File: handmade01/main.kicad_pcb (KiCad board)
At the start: 2 copper layers, 64.8 x 70.1 mm, 71 parts, among them CON1 MicroSD, CON2 MicroSD, J1 JACK_TRS_6PINS, P1 VOLUMN, P4 USB_OTG, P6 UART_DEBUG, Q1 1AM, SW1 Power, SW10 R, SW11 A, SW12 B, SW13 X, SW14 Y, SW2 Reset, SW3 UP, SW4 Down, SW5 Left, SW6 Right, SW7 Select, SW8 Start, SW9 L, U1 PCM5102A, U2 PAM8403, U3 IPS_2.4_240x320_ST7789V, U4 CM3354, U5 TPS71718

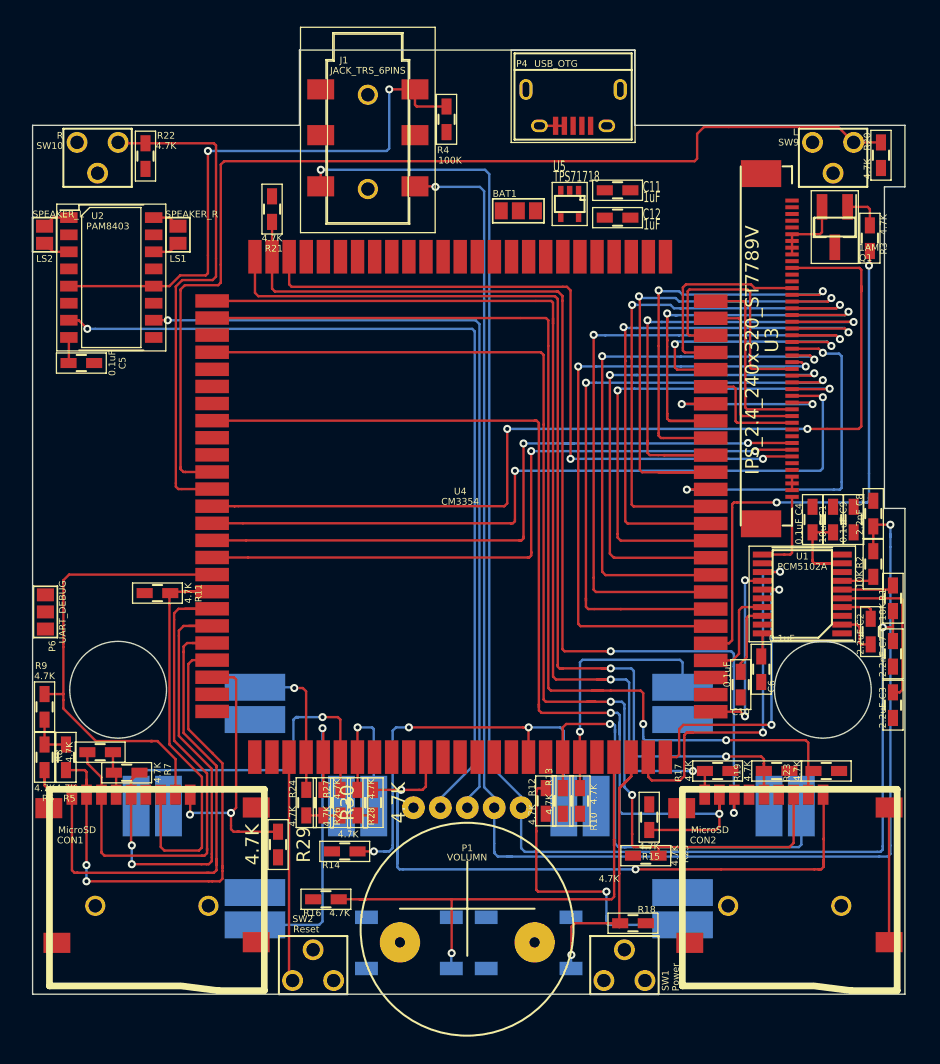
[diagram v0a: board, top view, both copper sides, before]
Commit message: 20171217
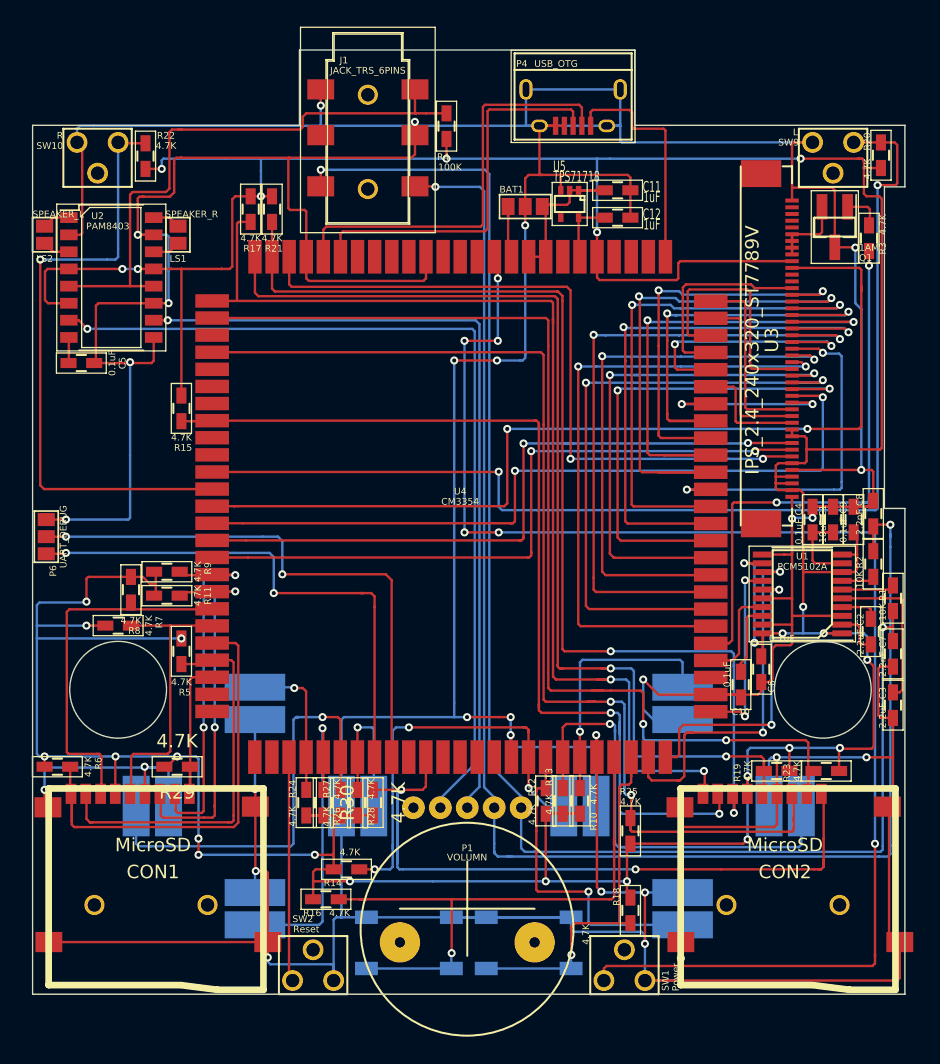
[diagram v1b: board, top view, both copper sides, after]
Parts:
- moved R17 54.2 mm to (126.7, 79.4), turned to 270 degrees
- moved R15 46.1 mm to (121.5, 94.2)
- moved R9 13.5 mm to (120.5, 106.3), turned to 0 degrees
- moved R8 12.3 mm to (117.8, 107.6), turned to 270 degrees
- moved R5 11.6 mm to (121.5, 112.2)
- moved R7 10.9 mm to (116.8, 110.3)
- moved R29 9.46 mm to (121.2, 120.8), turned to 180 degrees
- moved P6 5.59 mm to (111.5, 103.7)
- moved R25 2.17 mm to (154.9, 125.5), turned to 90 degrees
- moved R14 1.34 mm to (133.8, 128.4)
- moved R6 1.18 mm to (112.3, 120.8), turned to 0 degrees
- moved R18 0.97 mm to (154.9, 131.4), turned to 270 degrees
- moved R11 0.72 mm to (120.5, 108.1)
- moved BAT1 0.60 mm to (147.1, 79.2)
- moved R4 0.51 mm to (141.2, 73.2)
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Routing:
- net GND: track 28.6 -> 586.5 mm, vias 0 -> 29
- net +3.3V: track 14.4 -> 363.5 mm, vias 0 -> 29
- net POWER: track 0.00 -> 106.8 mm, vias 0 -> 6
- net UART_TX: track 0.00 -> 41.6 mm, vias 0 -> 2
- net UART_RX: track 0.00 -> 39.4 mm, vias 0 -> 2
- net USB_DM: track 0.00 -> 31.6 mm
- net USB_DP: track 0.00 -> 29.0 mm
- net +5V: track 0.00 -> 17.3 mm
- net SD0_CLK: track 35.6 -> 21.3 mm, vias 2 -> 0
- net SD0_CMD: track 39.8 -> 26.9 mm
- net BAT_+: track 0.00 -> 12.8 mm
- net SD0_DAT3: track 40.0 -> 28.8 mm, vias 2 -> 0
- net SD0_CD: track 21.4 -> 12.3 mm, vias 2 -> 0
- net SD0_DAT2: track 42.6 -> 34.2 mm
- net R: track 38.0 -> 46.1 mm, vias 0 -> 1
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
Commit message: 20171217
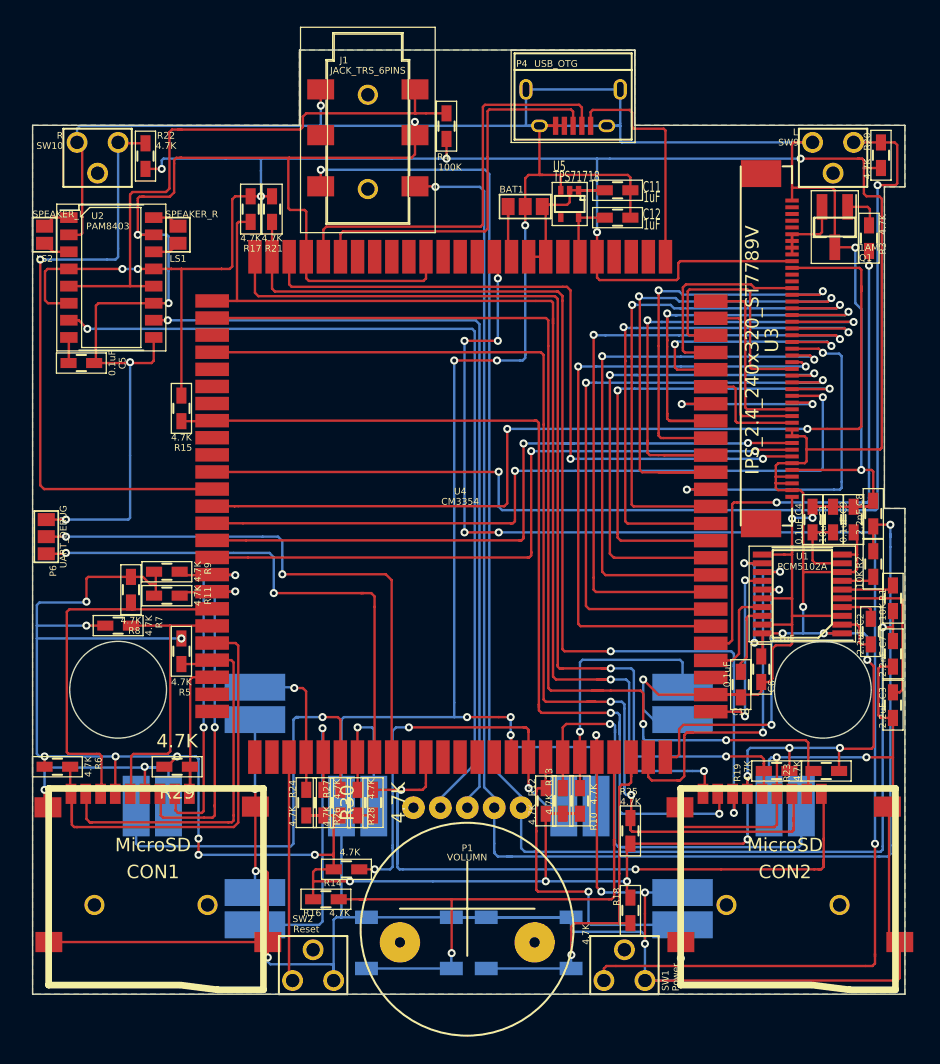
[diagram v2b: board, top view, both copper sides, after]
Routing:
- added copper zone on B.Cu, net GND
- added copper zone on F.Cu, net GND
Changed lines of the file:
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@@
   (page A4)
   (layers
-    (15 F.Cu signal)
-    (0 B.Cu signal)
-    (16 B.Adhes user)
-    (17 F.Adhes user)
-    (18 B.Paste user)
-    (19 F.Paste user)
-    (20 B.SilkS user)
-    (21 F.SilkS user)
-    (22 B.Mask user)
-    (23 F.Mask user)
-    (24 Dwgs.User user)
-    (25 Cmts.User user)
-    (26 Eco1.User user)
-    (27 Eco2.User user)
+    (15 F.Cu signal hide)
+    (0 B.Cu signal hide)
+    (16 B.Adhes user hide)
+    (17 F.Adhes user hide)
+    (18 B.Paste user hide)
+    (19 F.Paste user hide)
+    (20 B.SilkS user hide)
+    (21 F.SilkS user hide)
+    (22 B.Mask user hide)
+    (23 F.Mask user hide)
+    (24 Dwgs.User user hide)
+    (25 Cmts.User user hide)
+    (26 Eco1.User user hide)
+    (27 Eco2.User user hide)
     (28 Edge.Cuts user)
   )
@@
     (pad_to_mask_clearance 0)
     (aux_axis_origin 0 0)
-    (visible_elements 7FFFFFEF)
+    (visible_elements 7FFFFFFF)
     (pcbplotparams
       (layerselection 536838145)
@@
   (segment (start 134.62 122.494) (end 134.62 120.0731) (width 0.18) (layer F.Cu) (net 87))
   (segment (start 134.62 120.0731) (end 134.6098 120.0629) (width 0.18) (layer F.Cu) (net 87))
+  (zone (net 12) (net_name GND) (layer B.Cu) (hatch edge 0.508)
+    (connect_pads (clearance 0.18))
+    (min_thickness 0.18)
+    (fill (arc_segments 16) (thermal_gap 0.2) (thermal_bridge_width 0.2))
+    (polygon
+      (pts
+        (xy 175.26 137.668) (xy 110.49 137.668) (xy 110.49 73.152) (xy 130.302 73.152) (xy 130.302 67.564)
+        (xy 155.194 67.564) (xy 155.194 73.152) (xy 175.26 73.152) (xy 175.26 77.724) (xy 173.736 77.724)
+        (xy 173.736 101.6) (xy 175.26 101.6)
+      )
+    )
+  )
+  (zone (net 12) (net_name GND) (layer F.Cu) (hatch edge 0.508)
+    (connect_pads (clearance 0.18))
+    (min_thickness 0.18)
+    (fill (arc_segments 16) (thermal_gap 0.2) (thermal_bridge_width 0.2))
+    (polygon
+      (pts
+        (xy 175.26 137.668) (xy 110.49 137.668) (xy 110.49 73.152) (xy 130.302 73.152) (xy 130.302 67.564)
+        (xy 155.194 67.564) (xy 155.194 73.152) (xy 175.26 73.152) (xy 175.26 77.724) (xy 173.736 77.724)
+        (xy 173.736 101.6) (xy 175.26 101.6)
+      )
+    )
+  )
 )

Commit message: 20171217
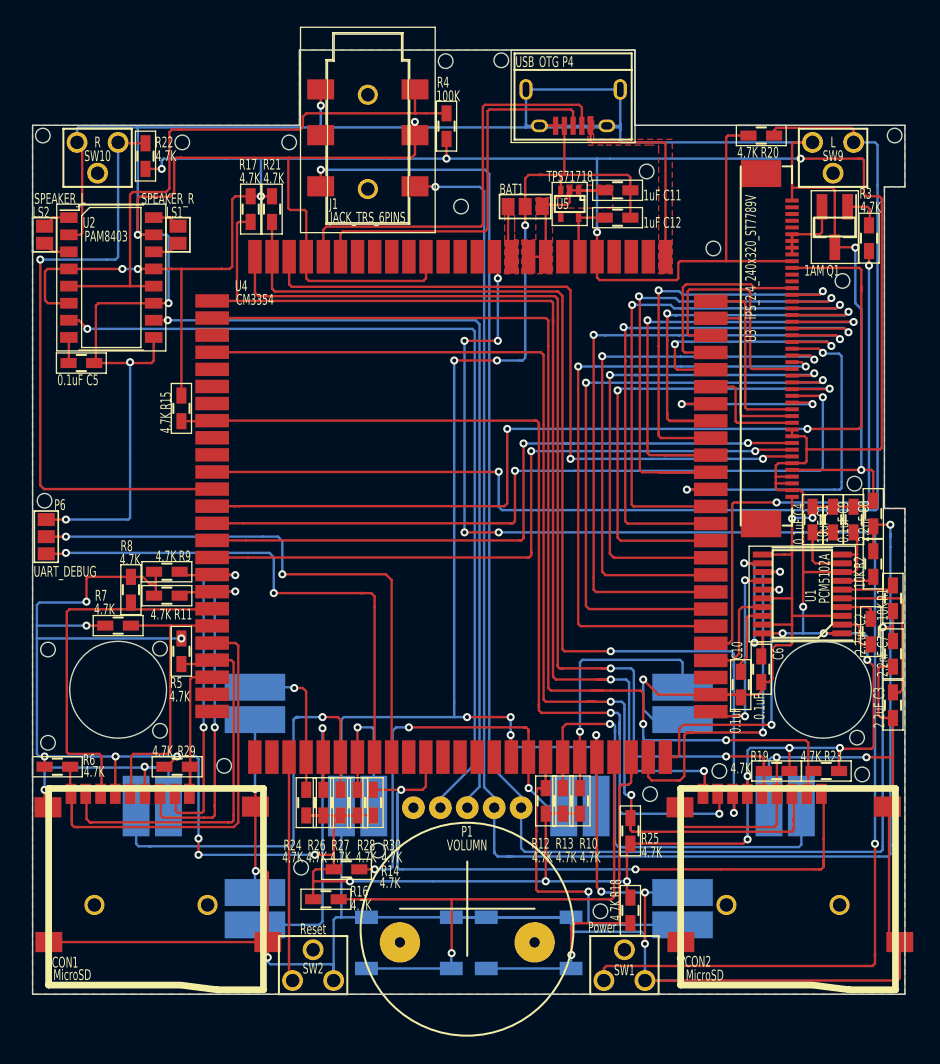
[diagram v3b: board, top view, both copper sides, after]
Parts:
- moved R20 9.01 mm to (164.6, 73.9), turned to 0 degrees
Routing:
- net GND: track 586.5 -> 600.7 mm
- net +3.3V: track 363.5 -> 373.1 mm
- net L: track 83.9 -> 88.4 mm, vias 2 -> 1
- net +5V: track 17.3 -> 15.2 mm
- added copper zone on F.Cu, net +5V
- added copper zone on F.Cu, net BAT_+
- added copper zone on F.Cu, net BAT_T
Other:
- outline, holes or cut-outs redrawn
- board text added: "Handmade01 Steward 20171217"
- board text removed: "Handmade01 Steward 20171212"
